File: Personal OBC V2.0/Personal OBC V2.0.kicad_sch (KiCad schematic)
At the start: 46 parts, among them J1 Screw_Terminal_01x02, J2 Screw_Terminal_01x04, J3 USB_B_Mini, J4 SWD Pins, Q1 SI7232DN-T1-GE3, U1 STM32F042G6Ux, U2 MS560702BA03-50, U3 AP2210N-3.3TRG1, U4 W25X40CLUXIG_TR, U5 LM293QT, Y1 ABM8G-16.000MHZ

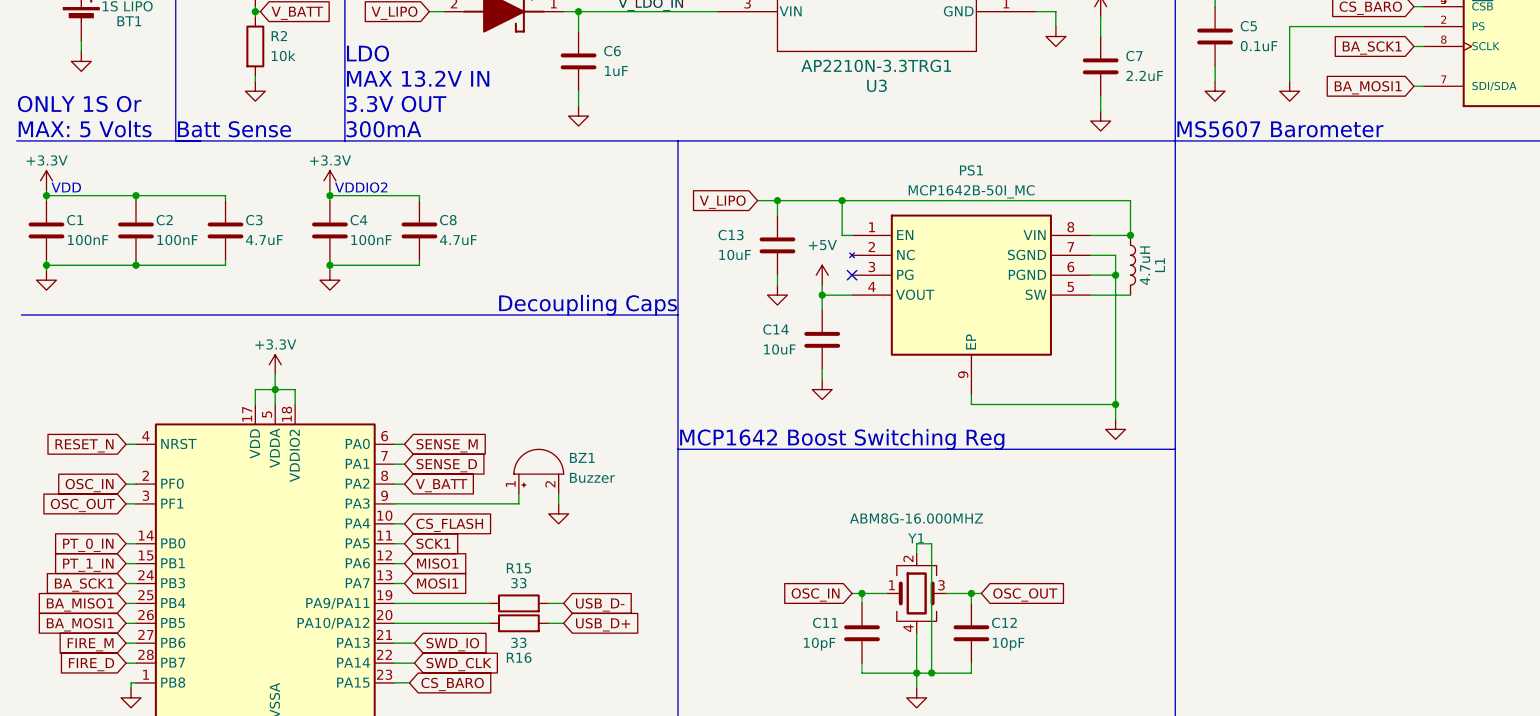
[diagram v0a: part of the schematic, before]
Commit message: Personal OBC Layout
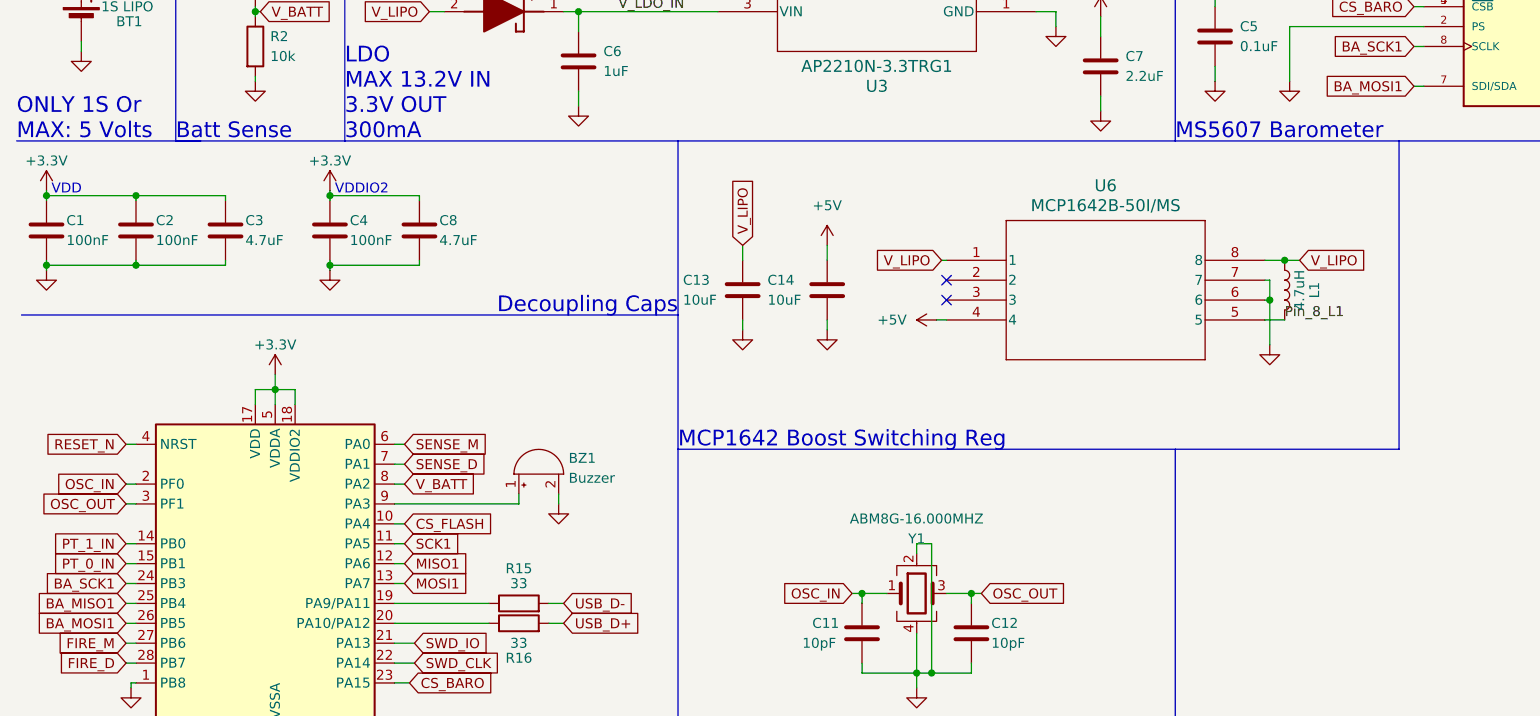
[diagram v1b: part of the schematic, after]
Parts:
- removed PS1: MCP1642B-50I_MC, MCP1642B-50I_MC:SON50P300X200X100-9N-D, symbol MCP1642B-50I_MC:MCP1642B-50I_MC
- added U6: MCP1642B-50I/MS, MCP1642B_50I_MS:MSOP8_MCP1642B-50I&slash_MS_MCH-L, symbol MCP1642B_50I_MS:MCP1642B-50I_MS
- BT1: footprint Connector_JST:JST_PH_S2B-PH-K_1x02_P2.00mm_Horizontal -> Connector_JST:JST_PH_B2B-PH-K_1x02_P2.00mm_Vertical
- C13, C14: footprint Capacitor_SMD:C_0603_1608Metric -> Capacitor_SMD:C_0603_1608Metric_Pad1.08x0.95mm_HandSolder
- C6, C7: footprint Capacitor_SMD:C_0402_1005Metric -> Capacitor_SMD:C_0402_1005Metric_Pad0.74x0.62mm_HandSolder
- J1: footprint TerminalBlock_TE-Connectivity:TerminalBlock_TE_282834-2_1x02_P2.54mm_Horizontal -> Conn_Screw_SMD:2_Pin_Conn
- J2: value Screw_Terminal_01x04 -> Screw_Terminal_01x08; footprint TerminalBlock_TE-Connectivity:TerminalBlock_TE_282834-8_1x08_P2.54mm_Horizontal -> Conn_Screw_SMD:8_Pin_Conn
- J4: footprint Connector_PinHeader_2.54mm:PinHeader_1x04_P2.54mm_Vertical -> Conn_Screw_SMD:4_Pin_Conn
- L1: footprint Inductor_SMD:L_1008_2520Metric -> Inductor_SMD:L_1008_2520Metric_Pad1.43x2.20mm_HandSolder
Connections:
- net +5V: now also U6.4
- net GND: now also U6.6, U6.7
- net PT_0_IN: now also U1.15 (PB1); no longer U1.14 (PB0)
- net PT_1_IN: now also U1.14 (PB0); no longer U1.15 (PB1)
- net V_LIPO: now also U6.1, U6.8
- net Pin_8_L1: now reaches L1.2
- net Pin_8_L1: now also U6.5
- no-connect marks 8 -> 9
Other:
- moved on the sheet: C13, C14, L1
